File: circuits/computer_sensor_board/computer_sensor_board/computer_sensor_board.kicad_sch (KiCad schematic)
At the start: 13 parts, among them J1 Conn_Main_ADC, J2 Conn_Jetson, J3 USB_M5Stack_0, J4 USB_M5Stack_1, J5 Conn_VLP16, U1 TDN_5-2411WISM, U2 Teensy4.1, U3 MCP3425_DIP

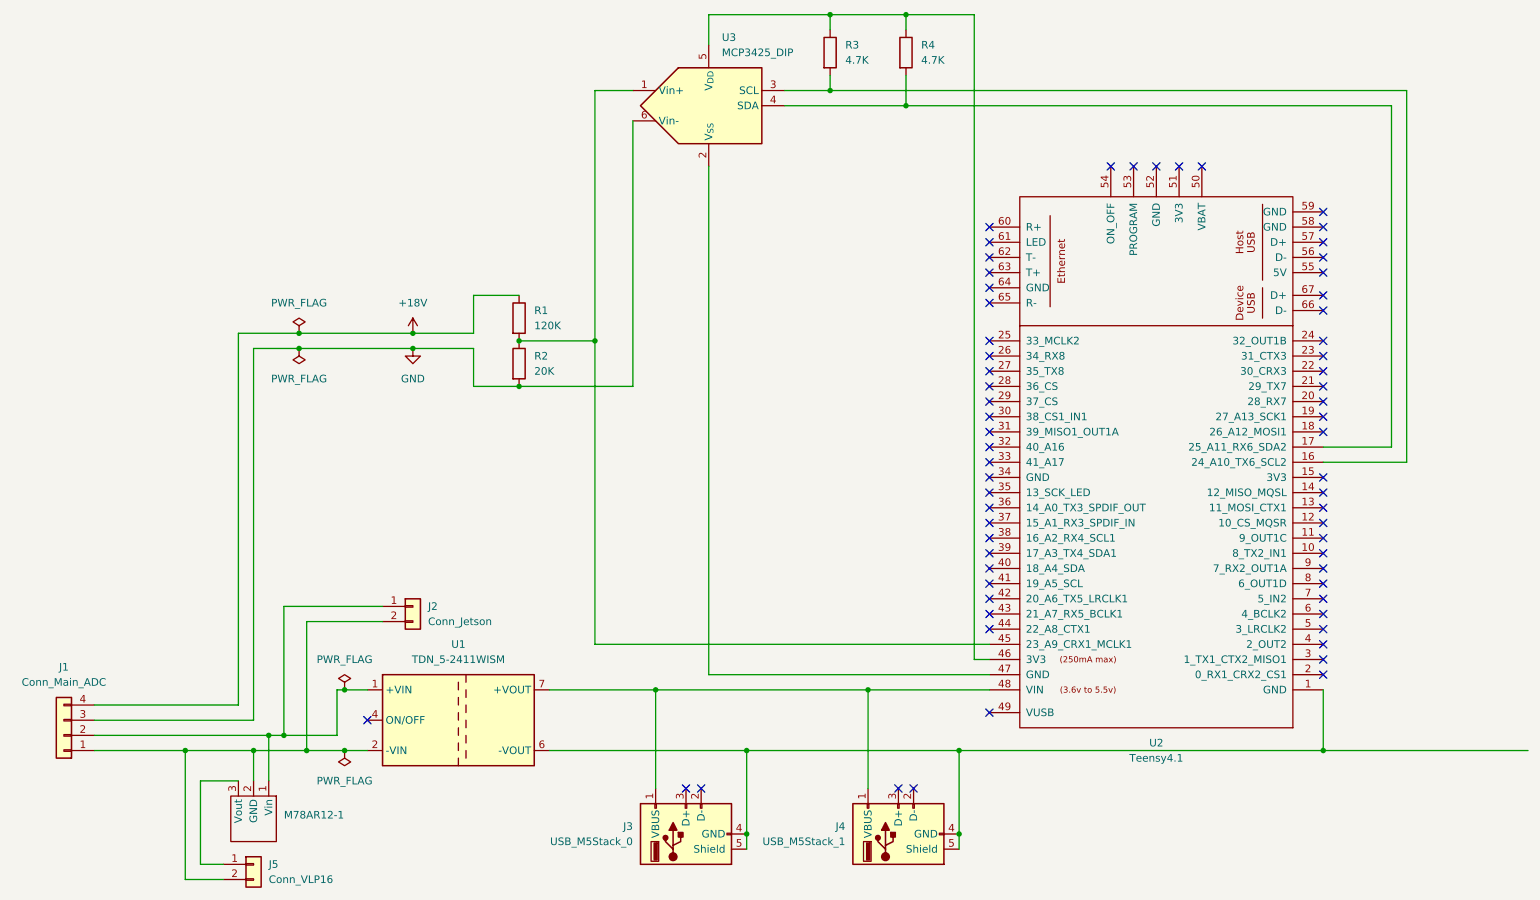
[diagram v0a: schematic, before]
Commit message: Feature/board design (#358)
* remove 19V line

Signed-off-by: Masaya Kataoka <ms.kataoka@gmail.com>

* design board

Signed-off-by: Masaya Kataoka <ms.kataoka@gmail.com>

* add description

Signed-off-by: Masaya Kataoka <ms.kataoka@gmail.com>

---------

Signed-off-by: Masaya Kataoka <ms.kataoka@gmail.com>
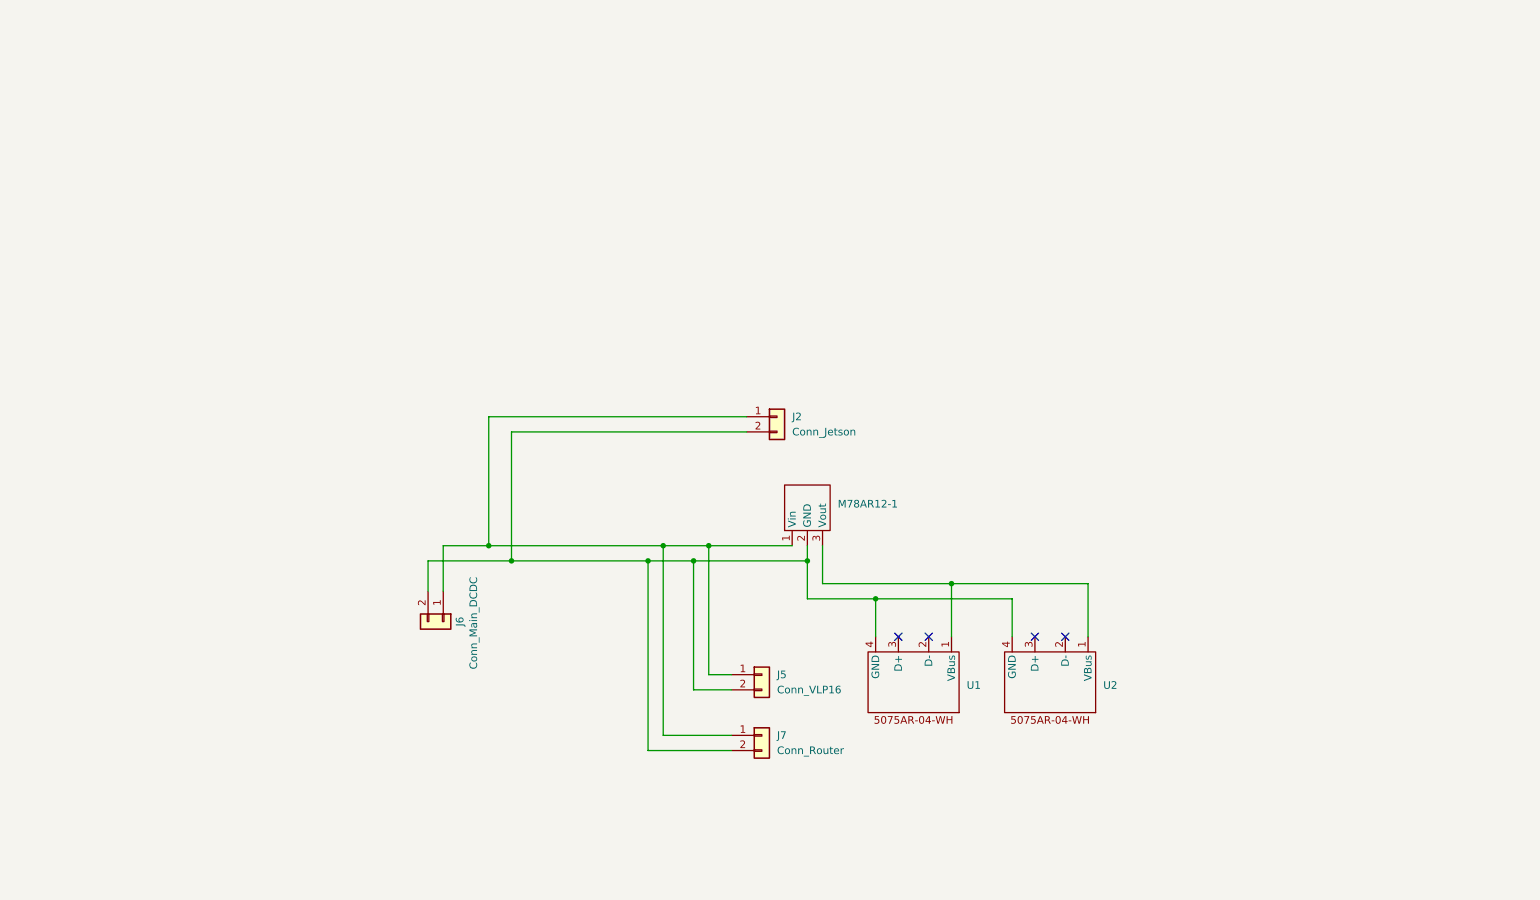
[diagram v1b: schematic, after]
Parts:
- removed J1: Conn_Main_ADC, symbol Connector_Generic:Conn_01x04
- removed J3: USB_M5Stack_0, symbol Connector:USB_A
- removed J4: USB_M5Stack_1, symbol Connector:USB_A
- removed R1: 120K, symbol Device:R
- removed R2: 20K, symbol Device:R
- removed R3, R4: 4.7K, symbol Device:R
- removed U1: TDN_5-2411WISM, Converter_DCDC:Converter_DCDC_TRACO_TDN_5-xxxxWISM_SMD, symbol Regulator_Switching:TDN_5-2411WISM
- removed U2: Teensy4.1, symbol teensy:Teensy4.1
- removed U3: MCP3425_DIP, Package_TO_SOT_SMD:SOT-23-6, symbol Analog_ADC:MCP3425Axx-xCH
- added J6: Conn_Main_DCDC, Connector_AMASS:AMASS_XT30PW-F_1x02_P2.50mm_Horizontal, symbol Connector_Generic:Conn_01x02
- added J7: Conn_Router, Connector_AMASS:AMASS_XT30PW-F_1x02_P2.50mm_Horizontal, symbol Connector_Generic:Conn_01x02
- added U1, U2: ~, 5075AR-04-WH:5075AR-04-WH, symbol 5075AR-04-WH:5075AR-04-WH
- J2, J5: footprint (none) -> Connector_AMASS:AMASS_XT30PW-F_1x02_P2.50mm_Horizontal
- M78AR12-1: footprint (none) -> M78AR15:M78AR15
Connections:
- net at J2.1 (Pin_1), M78AR12-1.1 (Vin): now also J5.1 (Pin_1), J6.1 (Pin_1), J7.1 (Pin_1)
- net at J2.2 (Pin_2), J5.2 (Pin_2), M78AR12-1.2 (GND): now also J6.2 (Pin_2), J7.2 (Pin_2), U1.4 (GND), U2.4 (GND)
- net at M78AR12-1.3 (Vout): now also U1.1 (VBus), U2.1 (VBus); no longer J5.1 (Pin_1)
- no-connect marks 65 -> 4
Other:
- moved on the sheet: J2, J5
